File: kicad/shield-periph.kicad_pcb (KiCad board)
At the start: 4 copper layers, 5 parts, among them J4 Fix, J5 Fix, J6 Fix, J7 Fix, U1 Conn_shield

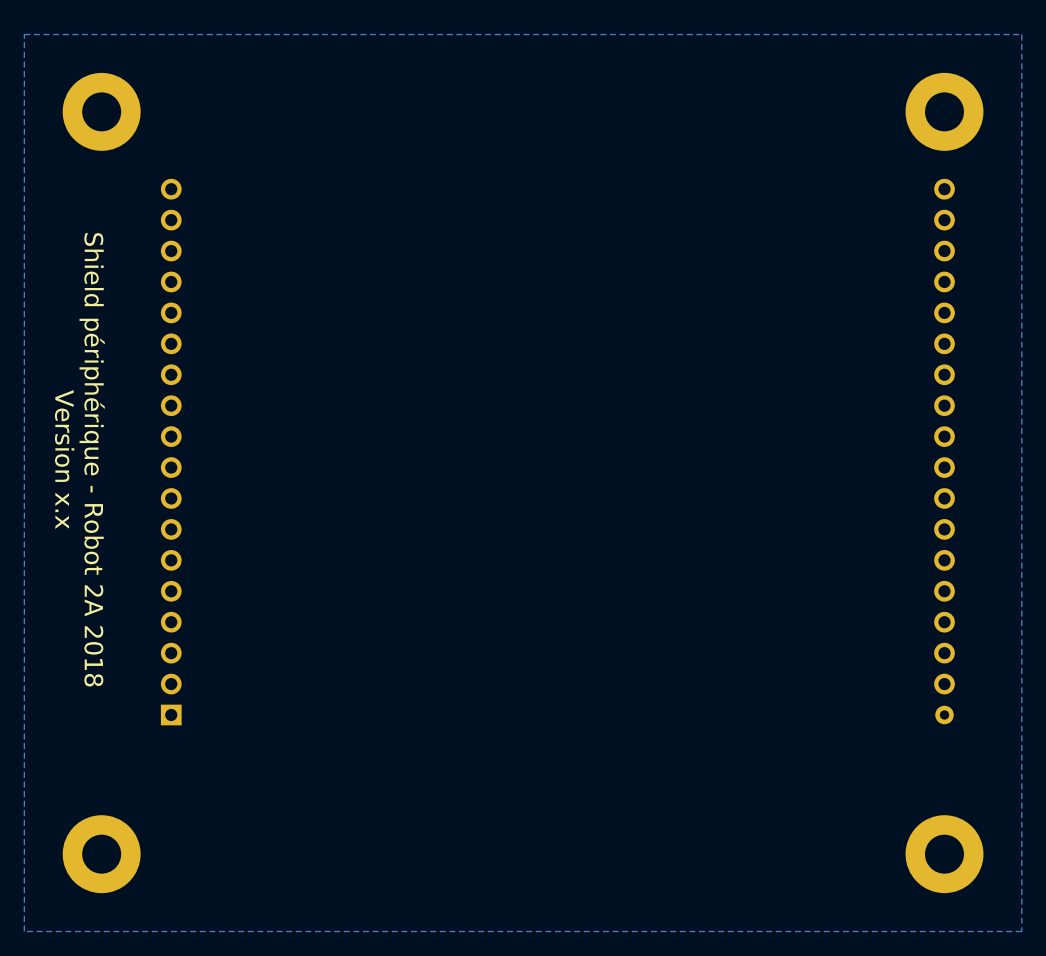
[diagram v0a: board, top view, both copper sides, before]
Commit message: Mise en conformité avec la carte periph
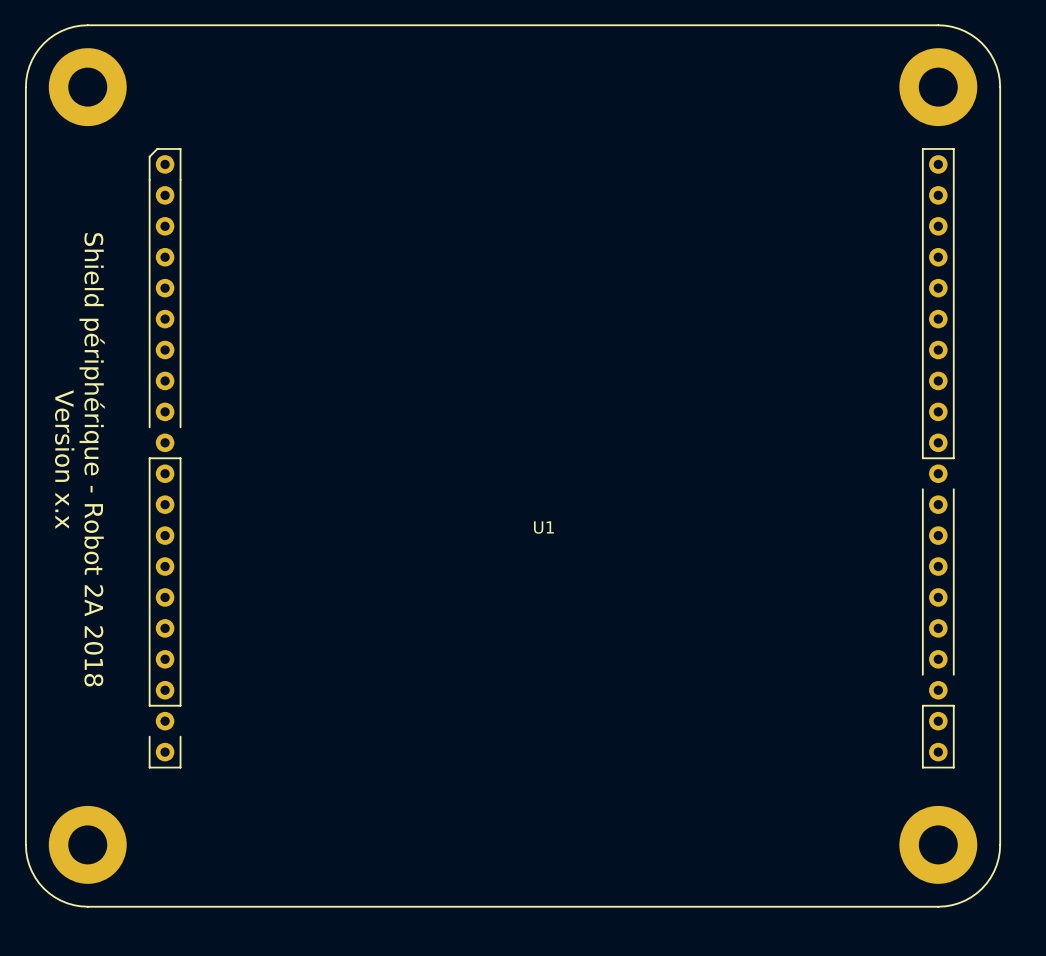
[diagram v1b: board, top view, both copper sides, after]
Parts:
- removed J4, J5, J6, J7: Fix, Mounting_Holes:MountingHole_3.2mm_M3_Pad
- U1: moved to F.Cu
- moved U1 3.09 mm to (46.5, 81.8), turned to 0 degrees
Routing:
- removed copper zone on In2.Cu, net +3V3
- removed copper zone on B.Cu, net GND
